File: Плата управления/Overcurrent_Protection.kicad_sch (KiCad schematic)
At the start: 15 parts, among them U5 LMV7239M5, U7 AD8210, U8 LMV324

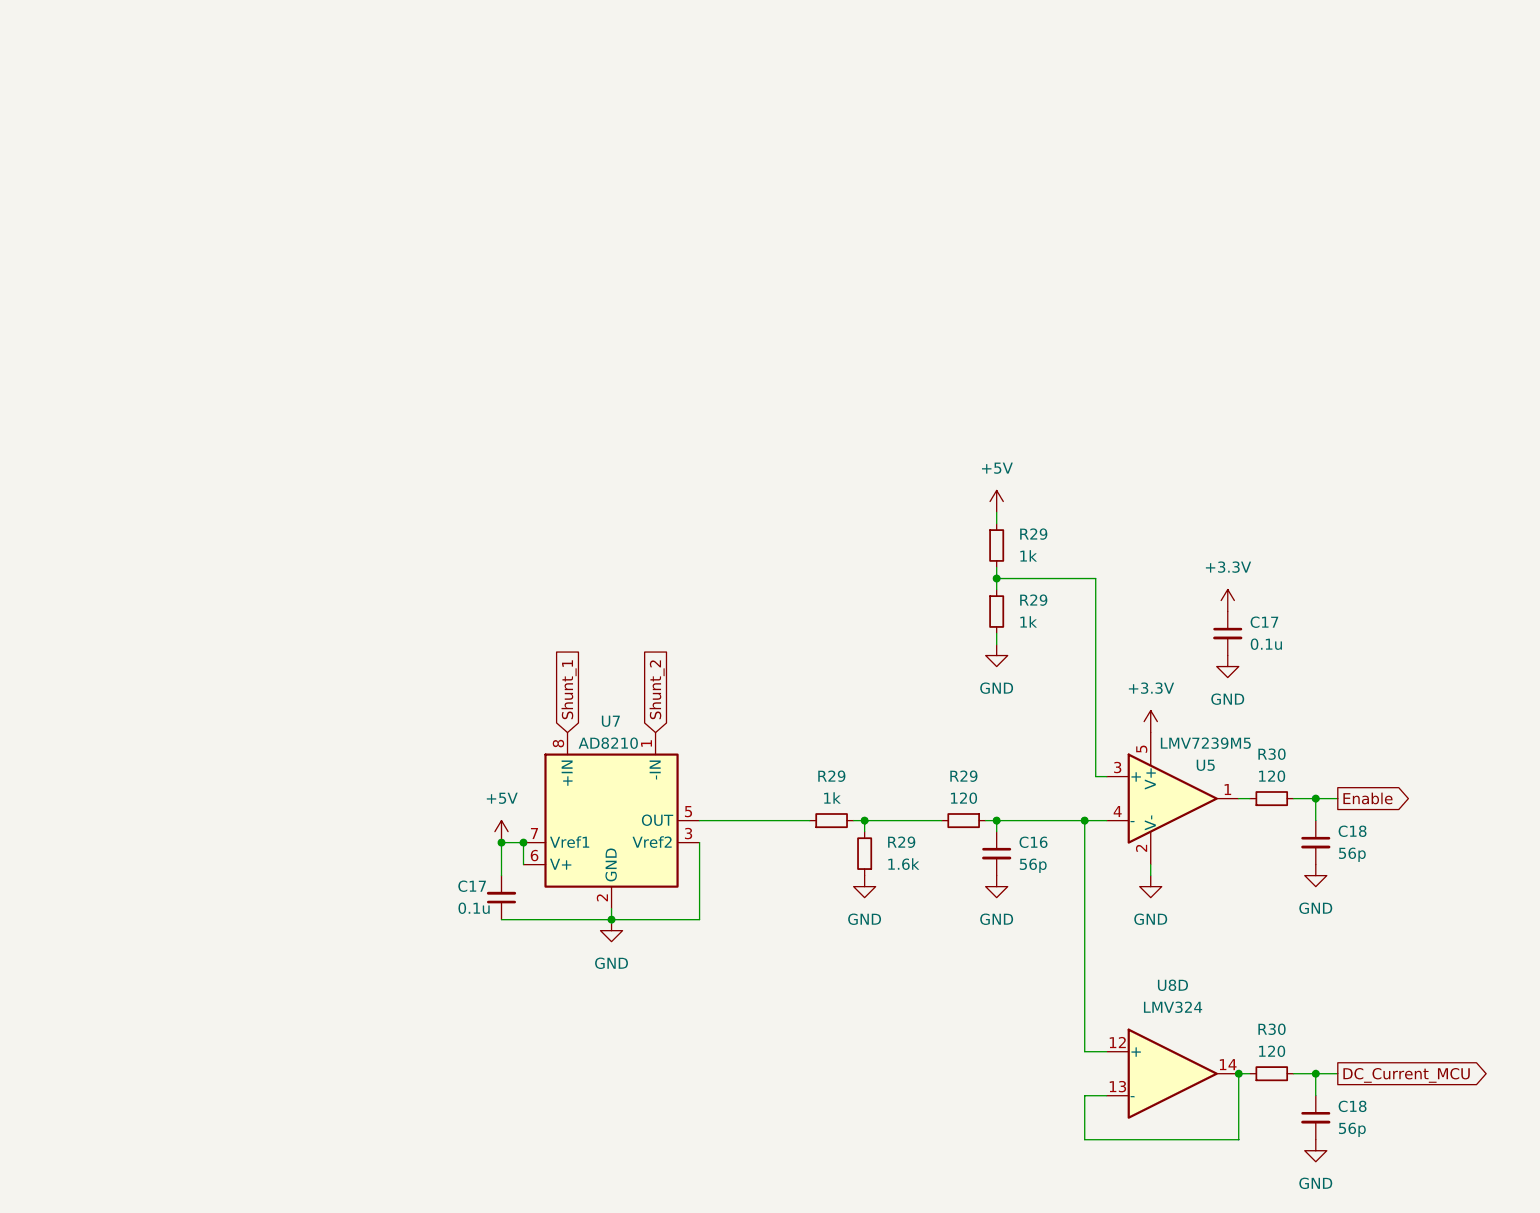
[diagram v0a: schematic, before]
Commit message: Привел в порядок схему
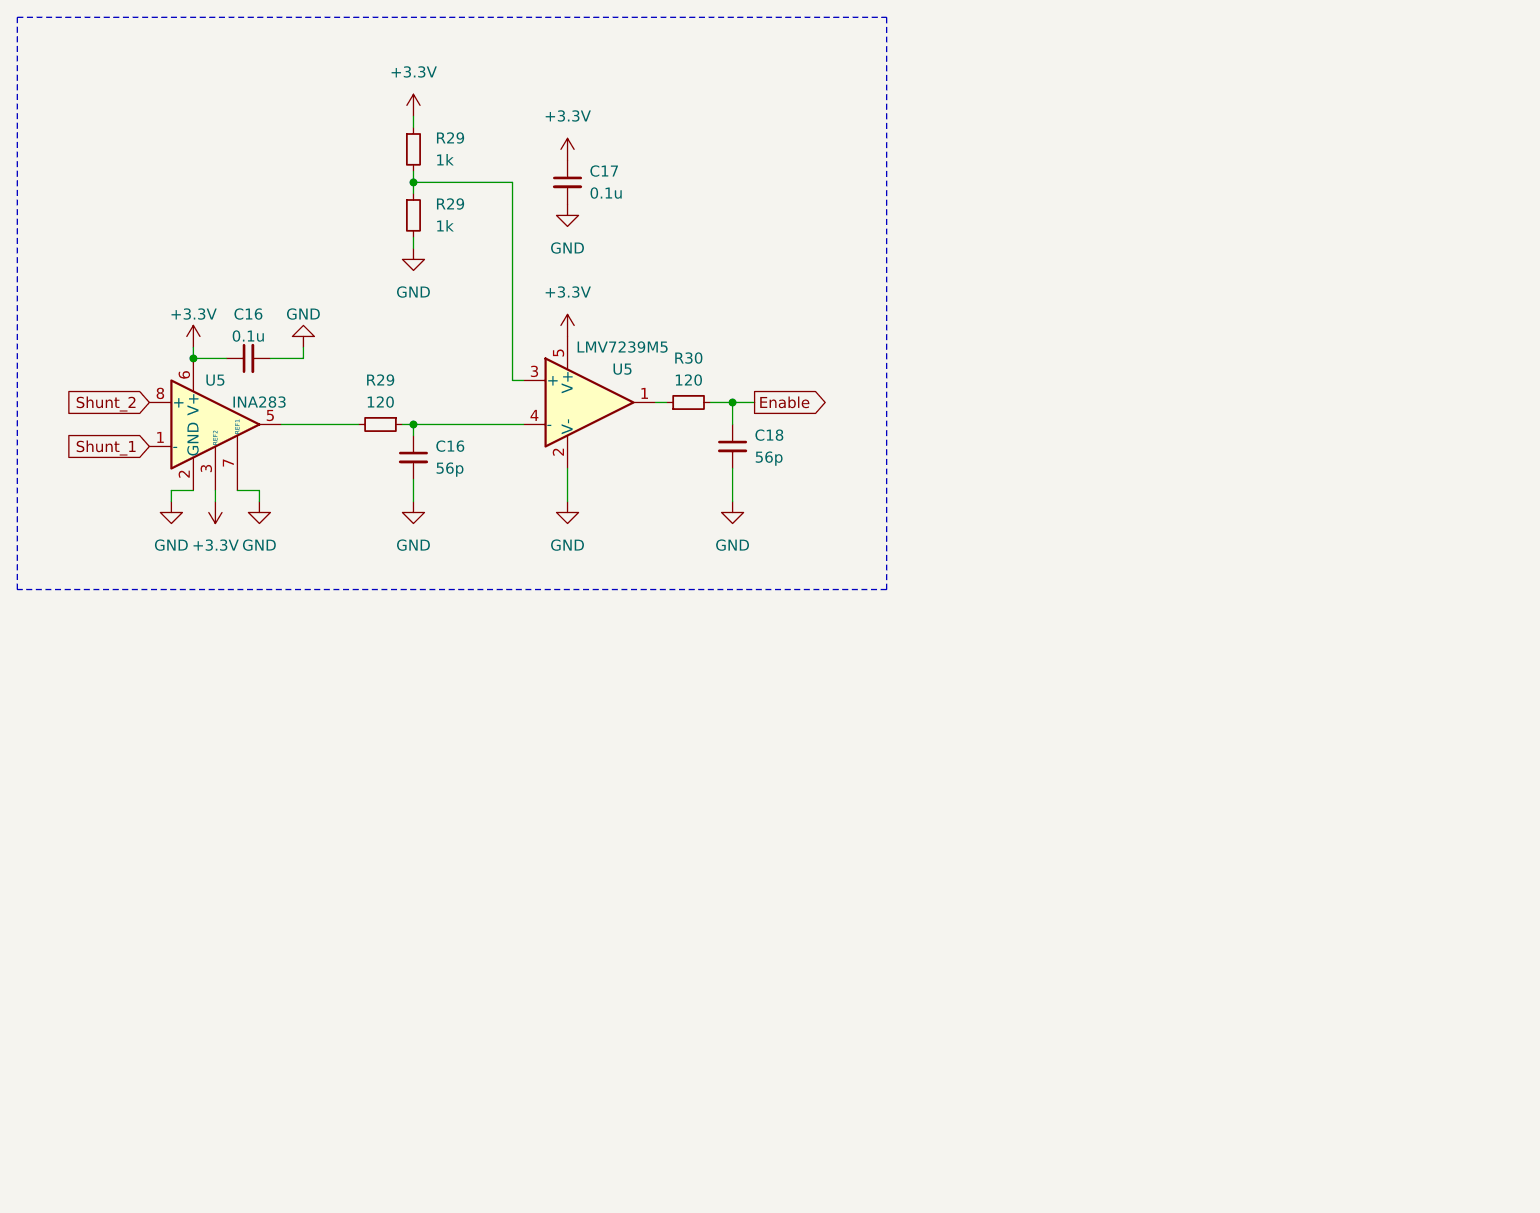
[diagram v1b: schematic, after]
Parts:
- removed C17: 0.1u, Capacitor_SMD:C_0603_1608Metric_Pad1.08x0.95mm_HandSolder, symbol Device:C_Small
- removed C18: 56p, Capacitor_SMD:C_0603_1608Metric_Pad1.08x0.95mm_HandSolder, symbol Device:C_Small
- removed R29: 1k, Resistor_SMD:R_0603_1608Metric_Pad0.98x0.95mm_HandSolder, symbol Device:R_Small
- removed R29: 1.6k, Resistor_SMD:R_0603_1608Metric_Pad0.98x0.95mm_HandSolder, symbol Device:R_Small
- removed R30: 120, Resistor_SMD:R_0603_1608Metric_Pad0.98x0.95mm_HandSolder, symbol Device:R_Small
- removed U7: AD8210, Package_SO:SOIC-8_3.9x4.9mm_P1.27mm, symbol Amplifier_Current:AD8210
- removed U8: LMV324, symbol Amplifier_Operational:LMV324
- added C16: 0.1u, Capacitor_SMD:C_0603_1608Metric_Pad1.08x0.95mm_HandSolder, symbol Device:C_Small
- added U5: INA283, Package_SO:SOIC-8_3.9x4.9mm_P1.27mm, symbol Amplifier_Current:INA283
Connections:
- net +5V is gone; now on net +3.3V: R29.1
- net +3.3V: now also C16.1, U5.3 (REF2), U5.6 (V+)
- net GND: now also C16.2, U5.2 (GND), U5.7 (REF1)
- net Shunt_1: now also U5.1 (-)
- net Shunt_2: now also U5.8 (+)
- net at R29.2: now also U5.5
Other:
- moved on the sheet: C16, C17, C18, R29, R30, U5
